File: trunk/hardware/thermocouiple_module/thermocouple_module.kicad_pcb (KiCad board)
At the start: 2 copper layers, 19 x 27.9 mm, 9 parts, among them P1 CONN_2, P2 CONN_1, P3 CONN_4, P4 CONN_2, U5 MAX31855KASA

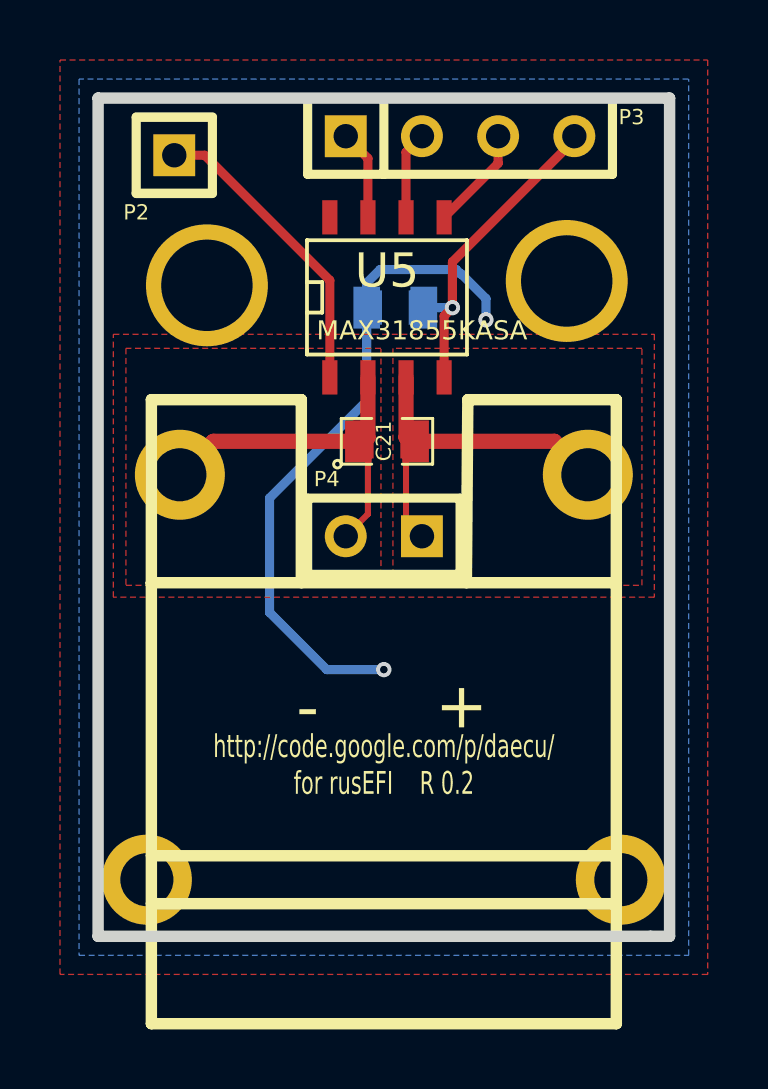
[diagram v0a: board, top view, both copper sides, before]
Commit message: 0.2
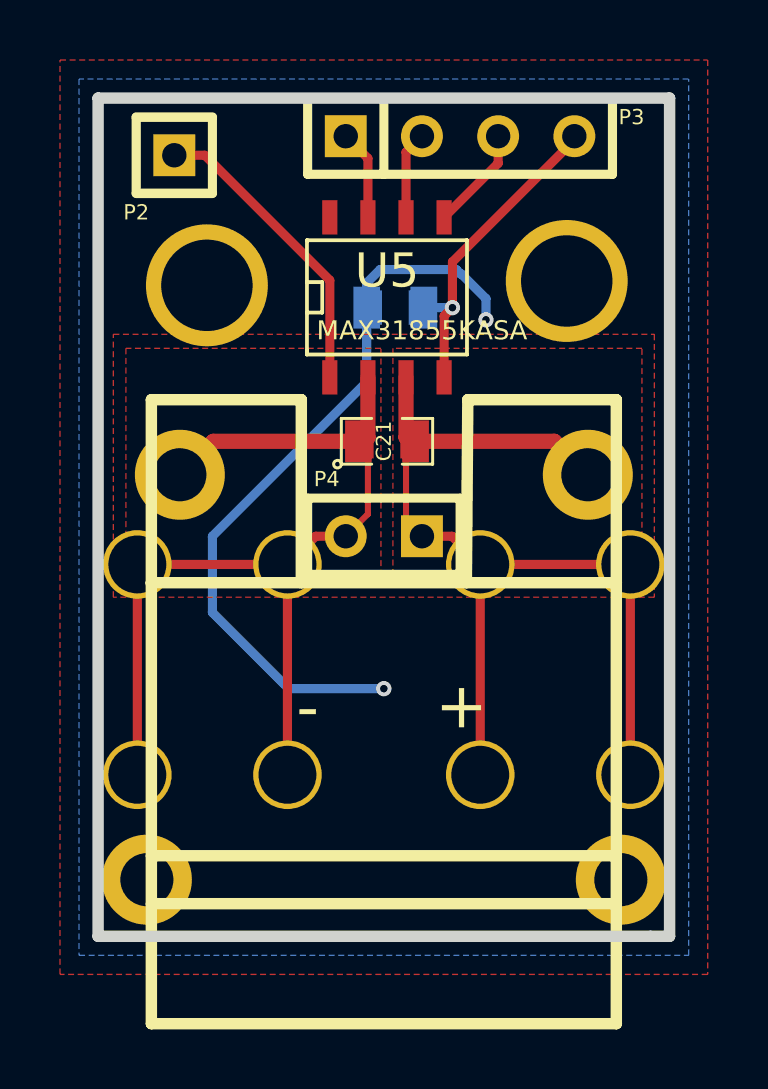
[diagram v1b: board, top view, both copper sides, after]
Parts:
- added P5: CONN_1, SCREW_TERM_534-7693, F.Cu at (99.1, 78.1)
- added P6: CONN_1, SCREW_TERM_534-7693, F.Cu at (110.5, 78.1)
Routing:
- net /TCPL-: track 14.4 -> 35.7 mm
- net /TCPL+: track 14.1 -> 35.5 mm
- net GND: track 32.5 -> 35.4 mm
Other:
- board text removed: "http://code.google.com/p/daecu/ for rusEFI"
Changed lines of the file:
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@@
 (kicad_pcb (version 3) (host pcbnew "(2013-07-07 BZR 4022)-stable")
   (general
-    (links 17)
+    (links 25)
     (no_connects 0)
     (area 93.7768 56.5658 124.877288 94.6912)
     (thickness 1.6002)
-    (drawings 15)
-    (tracks 44)
+    (drawings 14)
+    (tracks 54)
     (zones 0)
-    (modules 9)
+    (modules 11)
     (nets 8)
   )
-  (page A4)
+  (page A)
+  (title_block
+    (title "Thermocouple breakout")
+    (rev R0.2)
+    (company "rusEFI by DAECU")
+  )
   (layers
     (15 Front signal)
@@
       (outputformat 1)
       (mirror false)
-      (drillshape 1)
+      (drillshape 0)
       (scaleselection 1)
-      (outputdirectory gerbers/gerbers_Spin2/))
+      (outputdirectory thermocouple_gerbers))
   )
   (net 0 "")
@@
     )
   )
-  (gr_text "http://code.google.com/p/daecu/\nfor rusEFI    R 0.2" (at 104.775 81.28) (layer F.SilkS)
-    (effects (font (size 0.762 0.508) (thickness 0.127)))
-  )
-  (gr_text "http://code.google.com/p/daecu/\nfor rusEFI" (at 101.727 68.326 90) (layer B.SilkS)
+  (module SCREW_TERM_534-7693 (layer Front)
+    (at 99.06 78.105 180)
+    (fp_text reference P5 (at 0 -0.3175 180) (layer F.SilkS) hide
+      (effects (font (size 0.127 0.127) (thickness 0.00254)))
+    )
+    (fp_text value CONN_1 (at 0.09906 -0.8001 180) (layer F.SilkS) hide
+      (effects (font (size 0.127 0.127) (thickness 0.00254)))
+    )
+    (pad 1 thru_hole circle (at 2.5019 -3.5052 180) (size 2.286 2.286) (drill 1.9304)
+      (layers *.Cu *.Mask)
+      (net 5 /TCPL-)
+    )
+    (pad 1 thru_hole circle (at 2.5019 3.5052 180) (size 2.286 2.286) (drill 1.9304)
+      (layers *.Cu *.Mask)
+      (net 5 /TCPL-)
+    )
+    (pad 1 thru_hole circle (at -2.5019 3.5052 180) (size 2.286 2.286) (drill 1.9304)
+      (layers *.Cu *.Mask)
+      (net 5 /TCPL-)
+    )
+    (pad 1 thru_hole circle (at -2.5019 -3.5052 180) (size 2.286 2.286) (drill 1.9304)
+      (layers *.Cu *.Mask)
+      (net 5 /TCPL-)
+    )
+    (model 3D/screw_term_534-7693.wrl
+      (at (xyz 0 0 0.22))
+      (scale (xyz 10 10 10))
+      (rotate (xyz 270 0 90))
+    )
+  )
+  (module SCREW_TERM_534-7693 (layer Front)
+    (at 110.49 78.105 180)
+    (fp_text reference P6 (at 0 -0.3175 180) (layer F.SilkS) hide
+      (effects (font (size 0.127 0.127) (thickness 0.00254)))
+    )
+    (fp_text value CONN_1 (at 0.09906 -0.8001 180) (layer F.SilkS) hide
+      (effects (font (size 0.127 0.127) (thickness 0.00254)))
+    )
+    (pad 1 thru_hole circle (at 2.5019 -3.5052 180) (size 2.286 2.286) (drill 1.9304)
+      (layers *.Cu *.Mask)
+      (net 4 /TCPL+)
+    )
+    (pad 1 thru_hole circle (at 2.5019 3.5052 180) (size 2.286 2.286) (drill 1.9304)
+      (layers *.Cu *.Mask)
+      (net 4 /TCPL+)
+    )
+    (pad 1 thru_hole circle (at -2.5019 3.5052 180) (size 2.286 2.286) (drill 1.9304)
+      (layers *.Cu *.Mask)
+      (net 4 /TCPL+)
+    )
+    (pad 1 thru_hole circle (at -2.5019 -3.5052 180) (size 2.286 2.286) (drill 1.9304)
+      (layers *.Cu *.Mask)
+      (net 4 /TCPL+)
+    )
+    (model 3D/screw_term_534-7693.wrl
+      (at (xyz 0 0 0.22))
+      (scale (xyz 10 10 10))
+      (rotate (xyz 270 0 90))
+    )
+  )
+  (gr_text "http://code.google.com/p/daecu/\nfor rusEFI    R 0.2" (at 104.775 83.566) (layer B.SilkS)
     (effects (font (size 0.762 0.508) (thickness 0.127)) (justify mirror))
   )
@@
   (segment (start 108.585 60.325) (end 108.585 61.22924) (width 0.3048) (layer Front) (net 3))
   (segment (start 108.585 61.22924) (end 106.78414 63.0301) (width 0.3048) (layer Front) (net 3))
+  (segment (start 112.9919 74.5998) (end 107.9881 74.5998) (width 0.3048) (layer Front) (net 4))
+  (segment (start 112.9919 81.6102) (end 112.9919 74.5998) (width 0.3048) (layer Front) (net 4))
+  (segment (start 107.9881 81.6102) (end 107.9881 74.5998) (width 0.3048) (layer Front) (net 4))
+  (segment (start 106.045 73.66) (end 107.0483 73.66) (width 0.3048) (layer Front) (net 4))
+  (segment (start 107.0483 73.66) (end 107.9881 74.5998) (width 0.3048) (layer Front) (net 4))
   (segment (start 105.51414 68.3641) (end 105.51414 73.12914) (width 0.2032) (layer Front) (net 4))
   (segment (start 105.51414 73.12914) (end 106.045 73.66) (width 0.2032) (layer Front) (net 4))
@@
   (segment (start 105.64114 70.49516) (end 110.45952 70.49516) (width 0.508) (layer Front) (net 4))
   (segment (start 110.45952 70.49516) (end 111.57458 71.61022) (width 0.508) (layer Front) (net 4))
+  (segment (start 96.5581 74.5998) (end 101.5619 74.5998) (width 0.3048) (layer Front) (net 5))
+  (segment (start 101.5619 81.6102) (end 101.5619 74.5998) (width 0.3048) (layer Front) (net 5))
+  (segment (start 96.5581 81.6102) (end 96.5581 74.5998) (width 0.3048) (layer Front) (net 5))
+  (segment (start 103.505 73.66) (end 102.5017 73.66) (width 0.3048) (layer Front) (net 5))
+  (segment (start 102.5017 73.66) (end 101.5619 74.5998) (width 0.3048) (layer Front) (net 5))
   (segment (start 99.09048 70.49516) (end 97.97542 71.61022) (width 0.508) (layer Front) (net 5))
   (segment (start 104.11714 70.49516) (end 99.09048 70.49516) (width 0.508) (layer Front) (net 5))
@@
   (segment (start 106.78414 68.3641) (end 106.78414 66.31686) (width 0.3048) (layer Front) (net 6))
   (segment (start 106.78414 66.31686) (end 107.061 66.04) (width 0.3048) (layer Front) (net 6))
+  (segment (start 104.2035 66.04) (end 104.2035 68.5165) (width 0.3048) (layer Back) (net 7))
+  (via (at 104.775 78.74) (size 0.508) (layers Front Back) (net 7))
+  (segment (start 101.6 78.74) (end 104.775 78.74) (width 0.3048) (layer Back) (net 7))
+  (segment (start 99.06 76.2) (end 101.6 78.74) (width 0.3048) (layer Back) (net 7))
+  (segment (start 99.06 73.66) (end 99.06 76.2) (width 0.3048) (layer Back) (net 7))
+  (segment (start 104.2035 68.5165) (end 99.06 73.66) (width 0.3048) (layer Back) (net 7))
   (segment (start 107.3658 64.9224) (end 107.3404 64.9224) (width 0.3048) (layer Back) (net 7))
   (segment (start 107.3658 64.9224) (end 108.1786 65.7352) (width 0.3048) (layer Back) (net 7))
@@
   (segment (start 107.188 64.77) (end 104.648 64.77) (width 0.3048) (layer Back) (net 7))
   (segment (start 107.3404 64.9224) (end 107.188 64.77) (width 0.3048) (layer Back) (net 7))
-  (segment (start 104.2035 66.04) (end 104.2035 69.1515) (width 0.3048) (layer Back) (net 7))
-  (via (at 104.775 78.105) (size 0.508) (layers Front Back) (net 7))
-  (segment (start 102.87 78.105) (end 104.775 78.105) (width 0.3048) (layer Back) (net 7))
-  (segment (start 100.965 76.2) (end 102.87 78.105) (width 0.3048) (layer Back) (net 7))
-  (segment (start 100.965 72.39) (end 100.965 76.2) (width 0.3048) (layer Back) (net 7))
-  (segment (start 104.2035 69.1515) (end 100.965 72.39) (width 0.3048) (layer Back) (net 7))
   (segment (start 102.97414 68.3641) (end 102.97414 65.12814) (width 0.3048) (layer Front) (net 7))
   (segment (start 98.806 60.96) (end 97.79 60.96) (width 0.3048) (layer Front) (net 7))
